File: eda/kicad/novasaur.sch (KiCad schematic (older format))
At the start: 30 parts, among them SW2 RESET, U1 74F86, U10 74F574, U11 74F574, U12 PAL16R4, U2 74F32, U3 74F11, U4 74F139, U5 74F139, U6 74F157, U7 74F175, U8 74F574, U9 74F138, X1 33M

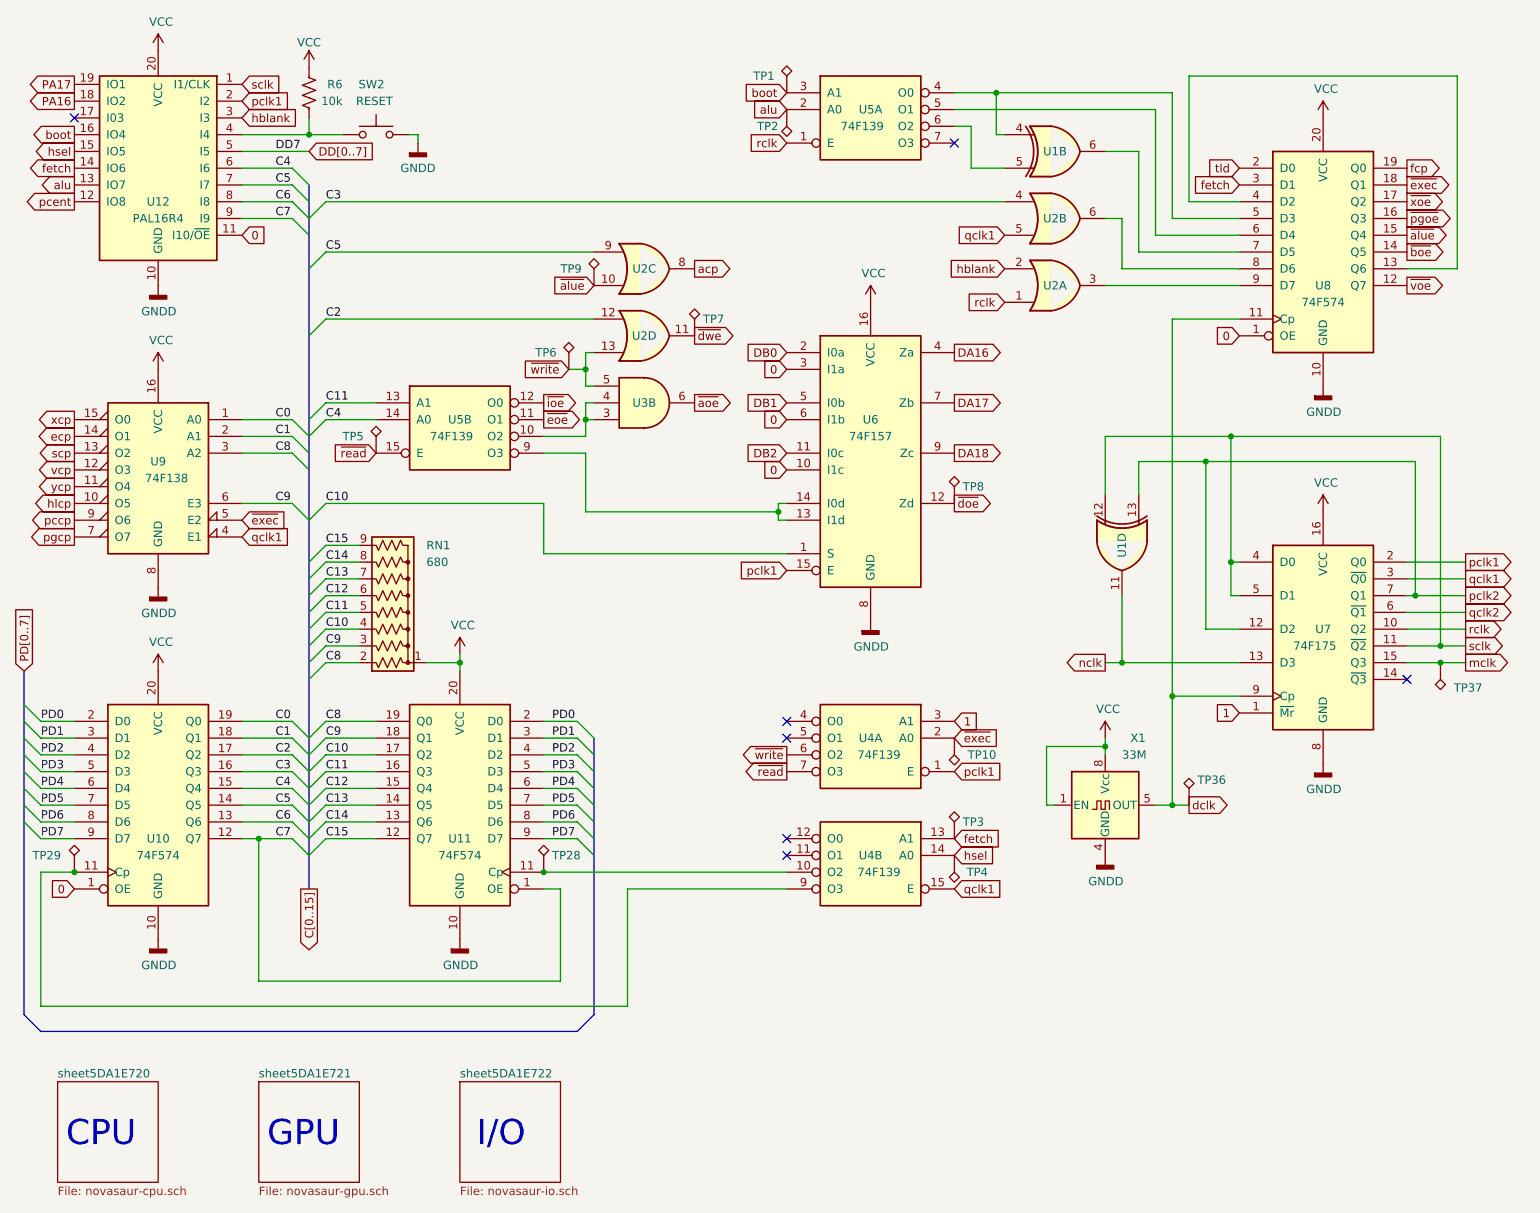
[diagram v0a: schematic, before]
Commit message: tweak schematic; new doc
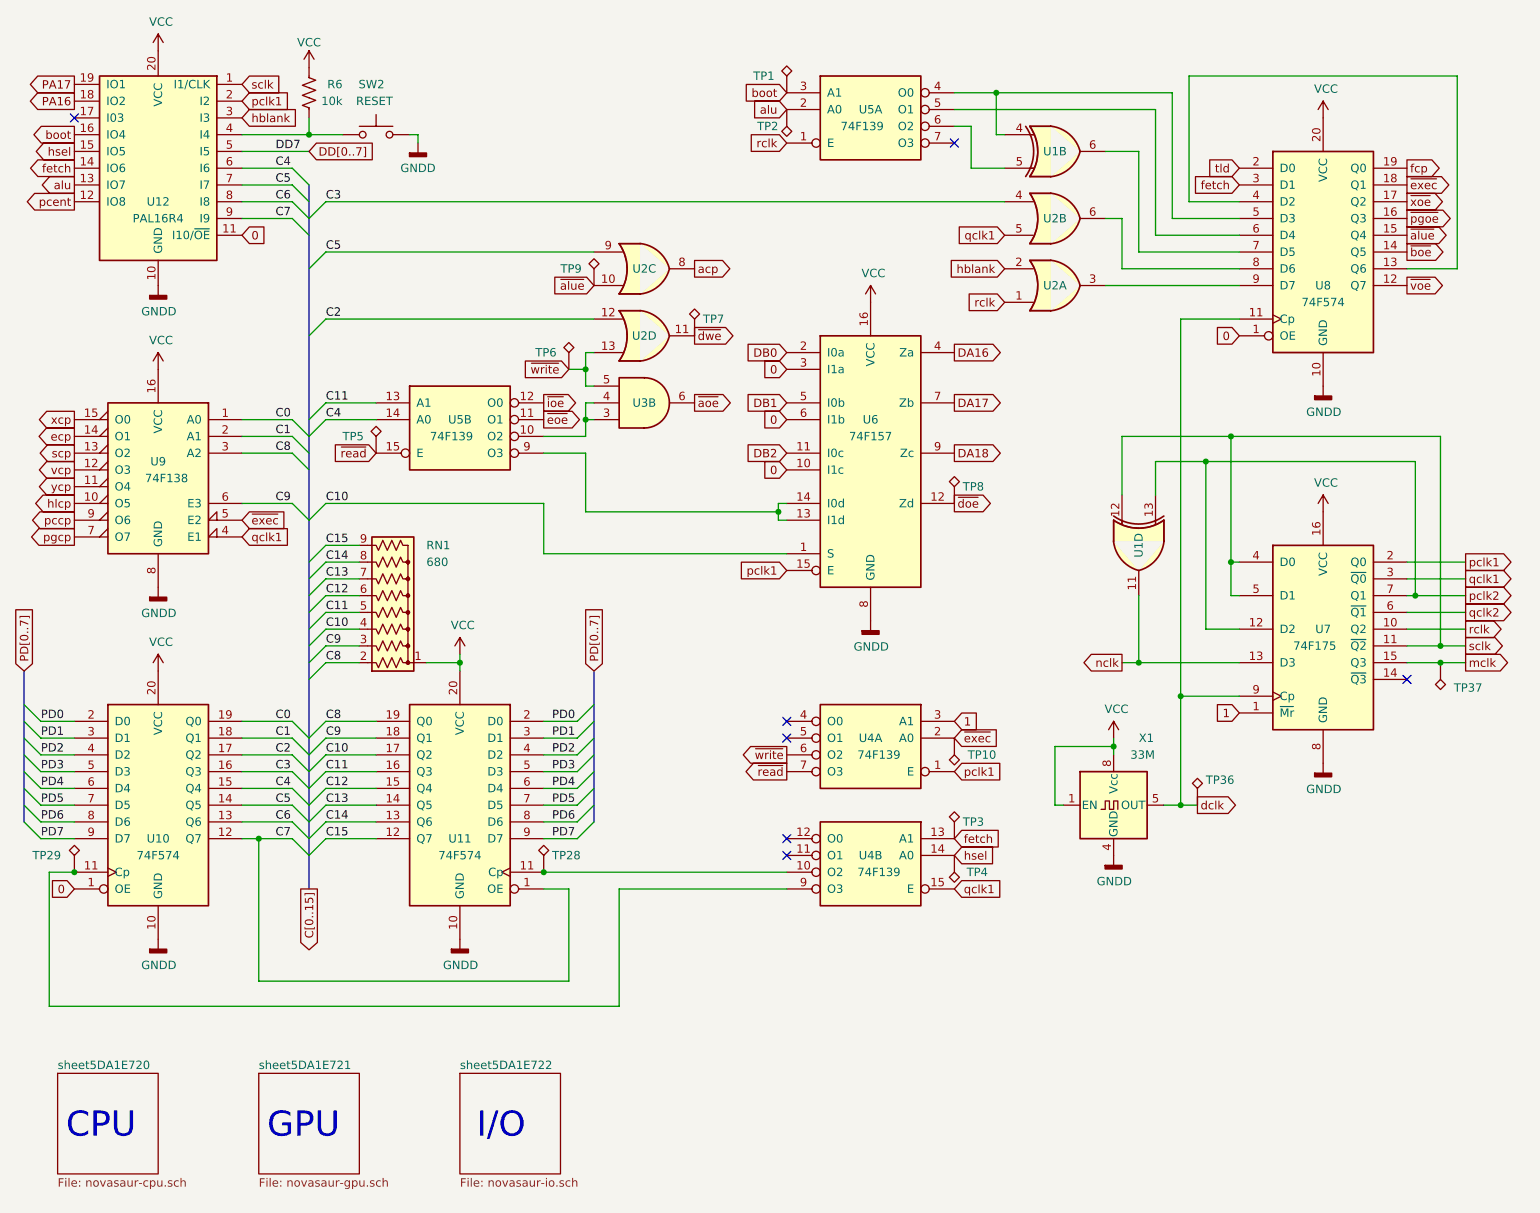
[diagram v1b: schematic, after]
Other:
- moved on the sheet: TP36, U1D, X1
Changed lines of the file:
@@
 Comment4 ""
 $EndDescr
-Wire Wire Line
-	4650 6000 4650 6700
-Wire Wire Line
-	4250 6000 4250 6550
 Text GLabel 1350 1800 0    50   Output ~ 0
 alu
-Wire Bus Line
-	1150 6850 4350 6850
 Wire Wire Line
 	2450 5700 2650 5700
@@
 	2350 1700 2650 1700
 NoConn ~ 1350 1400
-Entry Bus Bus
-	4350 6850 4450 6750
-Entry Bus Bus
-	1050 6750 1150 6850
 Text GLabel 2350 3900 2    50   Input ~ 0
 qclk1
@@
 Entry Wire Line
 	2650 1700 2750 1800
-Wire Wire Line
-	4250 6000 4150 6000
 $Comp
 L power:GNDD #PWR?
@@
 $EndComp
 Entry Wire Line
-	4450 5100 4350 5000
-Entry Wire Line
-	4450 5200 4350 5100
-Entry Wire Line
-	4450 5300 4350 5200
-Entry Wire Line
-	4450 5800 4350 5700
+	4450 4900 4350 5000
+Entry Wire Line
+	4450 5000 4350 5100
+Entry Wire Line
+	4450 5100 4350 5200
+Entry Wire Line
+	4450 5600 4350 5700
 Text Label 2550 5000 0    50   ~ 0
 C0
@@
 PD[0..7]
 Entry Wire Line
-	4450 5700 4350 5600
-Entry Wire Line
-	4450 5600 4350 5500
-Entry Wire Line
-	4450 5500 4350 5400
-Entry Wire Line
-	4450 5400 4350 5300
+	4450 5500 4350 5600
+Entry Wire Line
+	4450 5400 4350 5500
+Entry Wire Line
+	4450 5300 4350 5400
+Entry Wire Line
+	4450 5200 4350 5300
 Wire Wire Line
 	4150 5000 4350 5000
@@
 	2750 4750 2850 4650
 Wire Wire Line
-	1150 6700 4650 6700
-Wire Wire Line
-	2450 6550 4250 6550
-Wire Wire Line
 	2850 4250 3050 4250
 Wire Wire Line
@@
 Entry Wire Line
 	2850 3200 2750 3300
-Text Notes 3750 7550 0    150  ~ 0
-I/O
-Text Notes 2500 7550 0    150  ~ 0
-GPU
-Text Notes 1300 7550 0    150  ~ 0
-CPU
-$Sheet
-S 1250 7150 600  600
-U 5DA1E9BA
-F0 "sheet5DA1E720" 50
-F1 "novasaur-cpu.sch" 50
-$EndSheet
-$Sheet
-S 2450 7150 600  600
-U 5DA1E9BD
-F0 "sheet5DA1E721" 50
-F1 "novasaur-gpu.sch" 50
-$EndSheet
 Text Label 2850 3700 0    50   ~ 0
 C10
@@
 	1    0    0    -1
 $EndComp
-$Sheet
-S 3650 7150 600  600
-U 5DA1E9C0
-F0 "sheet5DA1E722" 50
-F1 "novasaur-io.sch" 50
-$EndSheet
 $Comp
 L power:VCC #PWR?
@@
 L Connector:TestPoint_Alt TP36
 U 1 1 5E2B88BD
-P 8000 5500
+P 8050 5500
 AR Path="/5E2B88BD" Ref="TP36"  Part="1"
 AR Path="/5DA1E9BA/5E2B88BD" Ref="TP?"  Part="1"
 AR Path="/5DA1E9BD/5E2B88BD" Ref="TP?"  Part="1"
 AR Path="/5DA1E9C0/5E2B88BD" Ref="TP?"  Part="1"
-F 0 "TP36" H 8050 5650 50  0000 L CNN
-F 1 "DCLK" H 7750 5650 50  0001 L CNN
-F 2 "TestPoint:TestPoint_THTPad_1.0x1.0mm_Drill0.5mm" H 8200 5500 50  0001 C CNN
-F 3 "~" H 8200 5500 50  0001 C CNN
-	1    8000 5500
-	1    0    0    -1
-$EndComp
-Wire Wire Line
-	7150 5500 7200 5500
-Wire Wire Line
-	7150 5150 7500 5150
+F 0 "TP36" H 8100 5650 50  0000 L CNN
+F 1 "DCLK" H 7800 5650 50  0001 L CNN
+F 2 "TestPoint:TestPoint_THTPad_1.0x1.0mm_Drill0.5mm" H 8250 5500 50  0001 C CNN
+F 3 "~" H 8250 5500 50  0001 C CNN
+	1    8050 5500
+	1    0    0    -1
+$EndComp
+Wire Wire Line
+	7200 5500 7250 5500
+Wire Wire Line
+	7200 5150 7550 5150
 Wire Wire Line
 	9500 3300 9500 4550
@@
 Wire Wire Line
 	8300 4050 8250 4050
-Text GLabel 7500 4650 0    50   Output ~ 0
+Text GLabel 7600 4650 0    50   Output ~ 0
 nclk
 NoConn ~ 9300 4750
 Wire Wire Line
-	7500 5150 7500 5100
-Connection ~ 7500 5150
-Wire Wire Line
-	7500 5200 7500 5150
+	7550 5150 7550 5100
+Connection ~ 7550 5150
+Wire Wire Line
+	7550 5200 7550 5150
 Wire Wire Line
 	9350 4250 9650 4250
@@
 L Oscillator:CXO_DIP8 X1
 U 1 1 5D9CA9D5
-P 7500 5500
-F 0 "X1" H 7650 5900 50  0000 L CNN
-F 1 "33M" H 7600 5800 50  0000 L CNN
-F 2 "Oscillator:Oscillator_DIP-8" H 7950 5150 50  0001 C CNN
-F 3 "http://cdn-reichelt.de/documents/datenblatt/B400/OSZI.pdf" H 7400 5500 50  0001 C CNN
-	1    7500 5500
+P 7550 5500
+F 0 "X1" H 7700 5900 50  0000 L CNN
+F 1 "33M" H 7650 5800 50  0000 L CNN
+F 2 "Oscillator:Oscillator_DIP-8" H 8000 5150 50  0001 C CNN
+F 3 "http://cdn-reichelt.de/documents/datenblatt/B400/OSZI.pdf" H 7450 5500 50  0001 C CNN
+	1    7550 5500
 	1    0    0    -1
 $EndComp
@@
 L power:GNDD #PWR?
 U 1 1 5D9CBE89
-P 7500 5800
+P 7550 5800
 AR Path="/5CDEEC9F/5D9CBE89" Ref="#PWR?"  Part="1"
 AR Path="/5DAA5CD8/5D9CBE89" Ref="#PWR?"  Part="1"
 AR Path="/5D9CBE89" Ref="#PWR0112"  Part="1"
-F 0 "#PWR0112" H 7500 5550 50  0001 C CNN
-F 1 "GNDD" H 7504 5645 50  0000 C CNN
-F 2 "" H 7500 5800 50  0001 C CNN
-F 3 "" H 7500 5800 50  0001 C CNN
-	1    7500 5800
+F 0 "#PWR0112" H 7550 5550 50  0001 C CNN
+F 1 "GNDD" H 7554 5645 50  0000 C CNN
+F 2 "" H 7550 5800 50  0001 C CNN
+F 3 "" H 7550 5800 50  0001 C CNN
+	1    7550 5800
 	1    0    0    -1
 $EndComp
@@
 L power:VCC #PWR0191
 U 1 1 5D9DED2A
-P 7500 5100
+P 7550 5100
 AR Path="/5D9DED2A" Ref="#PWR0191"  Part="1"
 AR Path="/5DAA5CD8/5D9DED2A" Ref="#PWR?"  Part="1"
-F 0 "#PWR0191" H 7500 4950 50  0001 C CNN
-F 1 "VCC" H 7517 5273 50  0000 C CNN
-F 2 "" H 7500 5100 50  0001 C CNN
-F 3 "" H 7500 5100 50  0001 C CNN
-	1    7500 5100
-	1    0    0    -1
-$EndComp
-Text GLabel 8000 5500 2    50   Output ~ 0
+F 0 "#PWR0191" H 7550 4950 50  0001 C CNN
+F 1 "VCC" H 7567 5273 50  0000 C CNN
+F 2 "" H 7550 5100 50  0001 C CNN
+F 3 "" H 7550 5100 50  0001 C CNN
+	1    7550 5100
+	1    0    0    -1
+$EndComp
+Text GLabel 8050 5500 2    50   Output ~ 0
 dclk
 $Comp
@@
 DB2
 Wire Wire Line
-	7600 4650 7600 4250
+	7700 4650 7700 4250
 $Comp
 L Connector:TestPoint_Alt TP10
@@
 $EndComp
 Wire Wire Line
-	7600 4650 7500 4650
-Connection ~ 7600 4650
+	7700 4650 7600 4650
+Connection ~ 7700 4650
 Text GLabel 6600 3100 2    50   Output ~ 0
 DA17
@@
 	8250 4050 8250 3300
 Wire Wire Line
-	8250 3300 9500 3300
-Wire Wire Line
 	8100 4450 8100 3450
 Connection ~ 8100 3450
 Wire Wire Line
 	8100 4450 8300 4450
-Wire Wire Line
-	8100 3450 9350 3450
 Connection ~ 8250 3300
 Wire Wire Line
-	7900 4850 8300 4850
-Wire Wire Line
-	7500 3650 7500 3300
-Wire Wire Line
-	7500 3300 8250 3300
-Wire Wire Line
-	7700 3650 7700 3450
-Wire Wire Line
-	7700 3450 8100 3450
-Wire Wire Line
-	7900 2600 8300 2600
+	7600 3650 7600 3300
+Wire Wire Line
+	7600 3300 8250 3300
+Wire Wire Line
+	7800 3650 7800 3450
+Wire Wire Line
+	7800 3450 8100 3450
 Wire Wire Line
 	4400 3750 5550 3750
 Wire Wire Line
 	2850 1900 6900 1900
-Wire Wire Line
-	4650 6000 5600 6000
-Wire Wire Line
-	7800 5500 7900 5500
-Connection ~ 7900 5500
-Wire Wire Line
-	7900 5500 8000 5500
 Wire Wire Line
 	4450 3200 4400 3200
@@
 	4400 2900 4400 2800
 Wire Wire Line
-	7150 5150 7150 5500
-Wire Wire Line
-	7900 4850 7900 5500
-Wire Wire Line
-	7600 4650 8300 4650
-Wire Wire Line
-	7900 4850 7900 2600
-Connection ~ 7900 4850
+	7200 5150 7200 5500
+Wire Wire Line
+	7700 4650 8300 4650
 Wire Wire Line
 	4400 3750 4400 3400
@@
 	1    0    0    -1
 $EndComp
-Wire Wire Line
-	1150 6700 1150 5900
-Wire Wire Line
-	1150 5900 1350 5900
 Connection ~ 1350 5900
 Wire Wire Line
@@
 L 74xx:74LS86 U1
 U 4 1 5F86670E
-P 7600 3950
+P 7700 3950
 AR Path="/5F86670E" Ref="U1"  Part="4"
 AR Path="/5DA1E9BD/5F86670E" Ref="U?"  Part="4"
 AR Path="/5DA1E9BA/5F86670E" Ref="U?"  Part="4"
-F 0 "U1" H 7600 3950 50  0000 C CNN
-F 1 "74F86" H 7600 4184 50  0001 C CNN
-F 2 "Package_DIP:DIP-14_W7.62mm_LongPads" H 7600 3950 50  0001 C CNN
-F 3 "74xx/74ls86.pdf" H 7600 3950 50  0001 C CNN
-	4    7600 3950
+F 0 "U1" H 7700 3950 50  0000 C CNN
+F 1 "74F86" H 7700 4184 50  0001 C CNN
+F 2 "Package_DIP:DIP-14_W7.62mm_LongPads" H 7700 3950 50  0001 C CNN
+F 3 "74xx/74ls86.pdf" H 7700 3950 50  0001 C CNN
+	4    7700 3950
 	0    -1   1    0
 $EndComp
@@
 Wire Wire Line
 	2750 1600 2350 1600
+Wire Wire Line
+	1200 5900 1200 6700
+Wire Wire Line
+	1200 5900 1350 5900
+Wire Wire Line
+	1200 6700 4600 6700
+Wire Wire Line
+	4600 6700 4600 6000
+Wire Wire Line
+	4600 6000 5600 6000
+Wire Wire Line
+	4300 6550 4300 6000
+Wire Wire Line
+	4150 6000 4300 6000
+Wire Wire Line
+	2450 6550 4300 6550
+Wire Wire Line
+	8100 3450 9350 3450
+Wire Wire Line
+	8250 3300 9500 3300
+Wire Wire Line
+	7950 5500 7950 4850
+Wire Wire Line
+	7950 2600 8300 2600
+Wire Wire Line
+	7950 4850 8300 4850
+Connection ~ 7950 4850
+Wire Wire Line
+	7950 4850 7950 2600
+Wire Wire Line
+	7850 5500 7950 5500
+Wire Wire Line
+	7950 5500 8050 5500
+Connection ~ 7950 5500
+Text GLabel 4450 4700 1    50   Input ~ 0
+PD[0..7]
+Text Notes 3750 7500 0    150  ~ 0
+I/O
+Text Notes 2500 7500 0    150  ~ 0
+GPU
+Text Notes 1300 7500 0    150  ~ 0
+CPU
+$Sheet
+S 1250 7100 600  600
+U 5DA1E9BA
+F0 "sheet5DA1E720" 50
+F1 "novasaur-cpu.sch" 50
+$EndSheet
+$Sheet
+S 2450 7100 600  600
+U 5DA1E9BD
+F0 "sheet5DA1E721" 50
+F1 "novasaur-gpu.sch" 50
+$EndSheet
+$Sheet
+S 3650 7100 600  600
+U 5DA1E9C0
+F0 "sheet5DA1E722" 50
+F1 "novasaur-io.sch" 50
+$EndSheet
 Wire Bus Line
-	4450 5100 4450 6750
+	4450 4700 4450 5600
 Wire Bus Line
-	1050 4700 1050 6750
+	1050 4700 1050 5600
 Wire Bus Line
 	2750 1800 2750 6000
